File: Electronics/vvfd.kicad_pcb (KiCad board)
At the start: 2 copper layers, 95 x 95 mm, 70 parts, among them J1 USB_C_Receptacle_USB2.0_14P, J2 Conn_01x02_Pin, J3 Conn_02x05_Counter_Clockwise, J4 Conn_02x05_Counter_Clockwise, J5 Conn_02x05_Counter_Clockwise, J6 Conn_01x08_Pin, J7 Conn_01x08_Pin, J8 Conn_01x08_Pin, J9 Conn_01x08_Pin, Q1 RFD14N05L, Q2 RFD14N05L, Q3 RFD14N05L, Q4 RFD14N05L, Q5 RFD14N05L, Q6 RFD14N05L, U1 MC34063AD, U10 TBD62783A, U2 TLV274, U3 74HC595, U4 TBD62783A, U5 74HC595, U6 TBD62783A, U7 74HC595, U8 TBD62783A, U9 74HC595

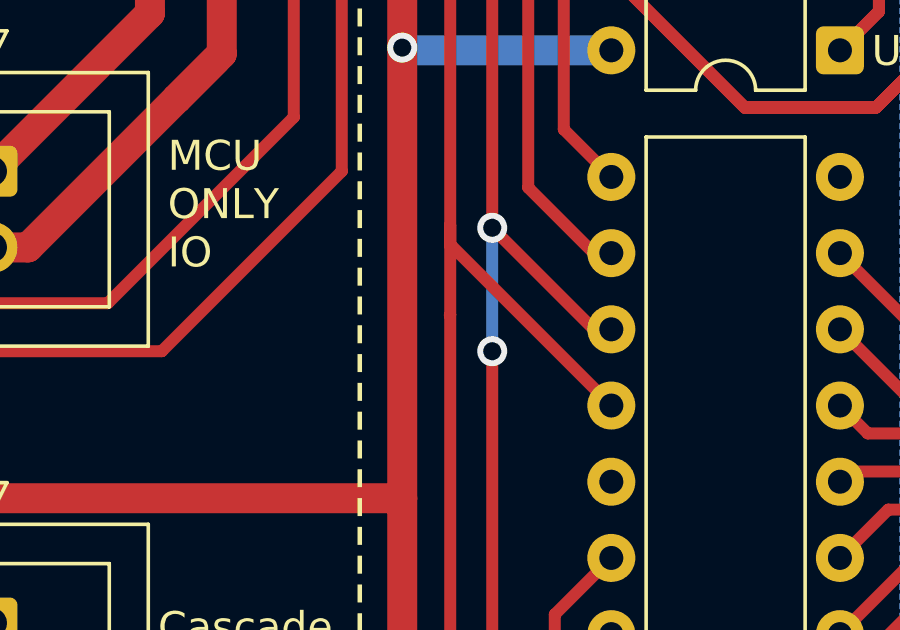
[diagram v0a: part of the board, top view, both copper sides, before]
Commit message: Fixed ERC and DRC
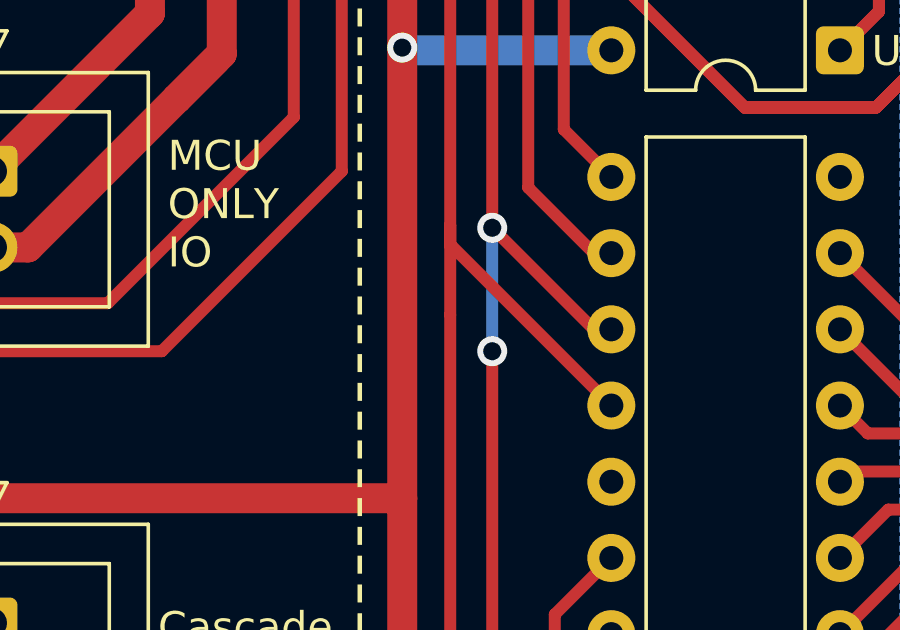
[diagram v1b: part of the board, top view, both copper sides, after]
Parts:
- Q1, Q2, Q3, Q4, Q5, Q6: value RFD14N05L -> IRLU014PBF
